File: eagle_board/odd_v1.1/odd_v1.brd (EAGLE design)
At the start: 100 x 40.6 mm, 17 parts

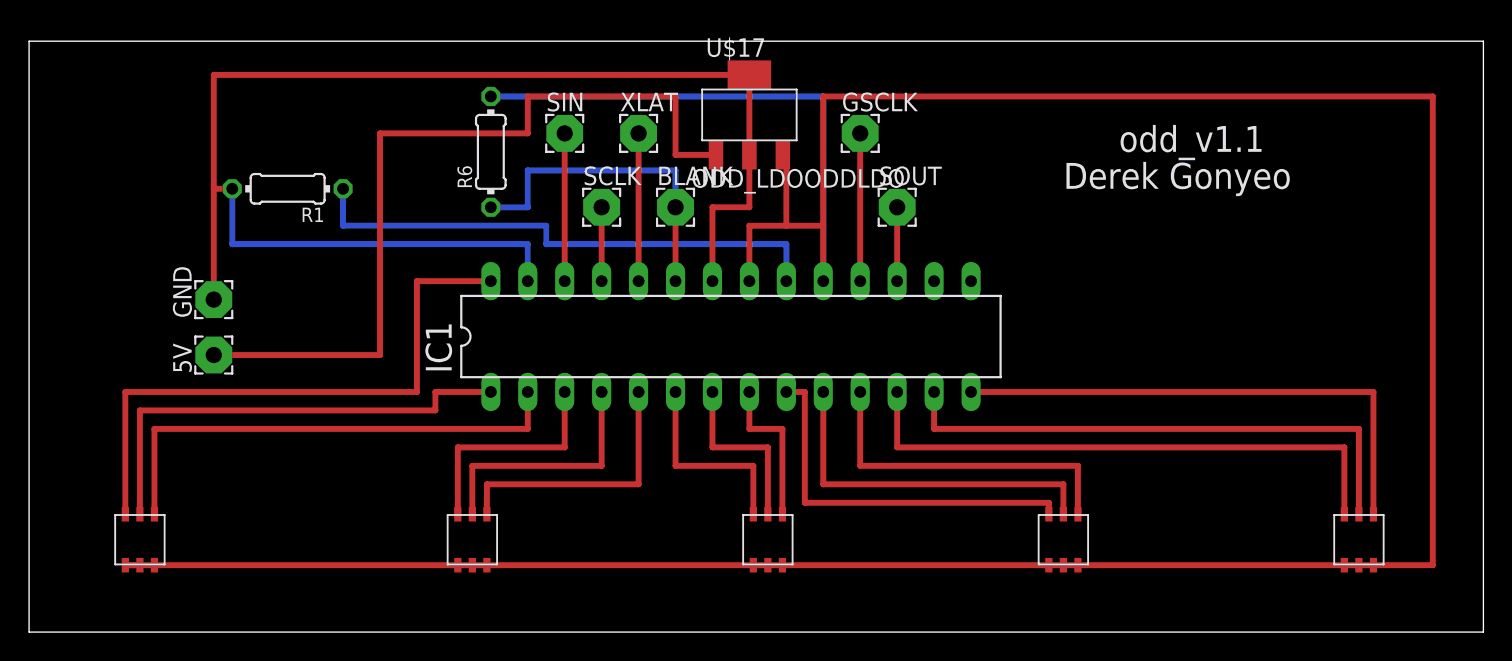
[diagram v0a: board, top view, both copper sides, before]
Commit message: Small changes.
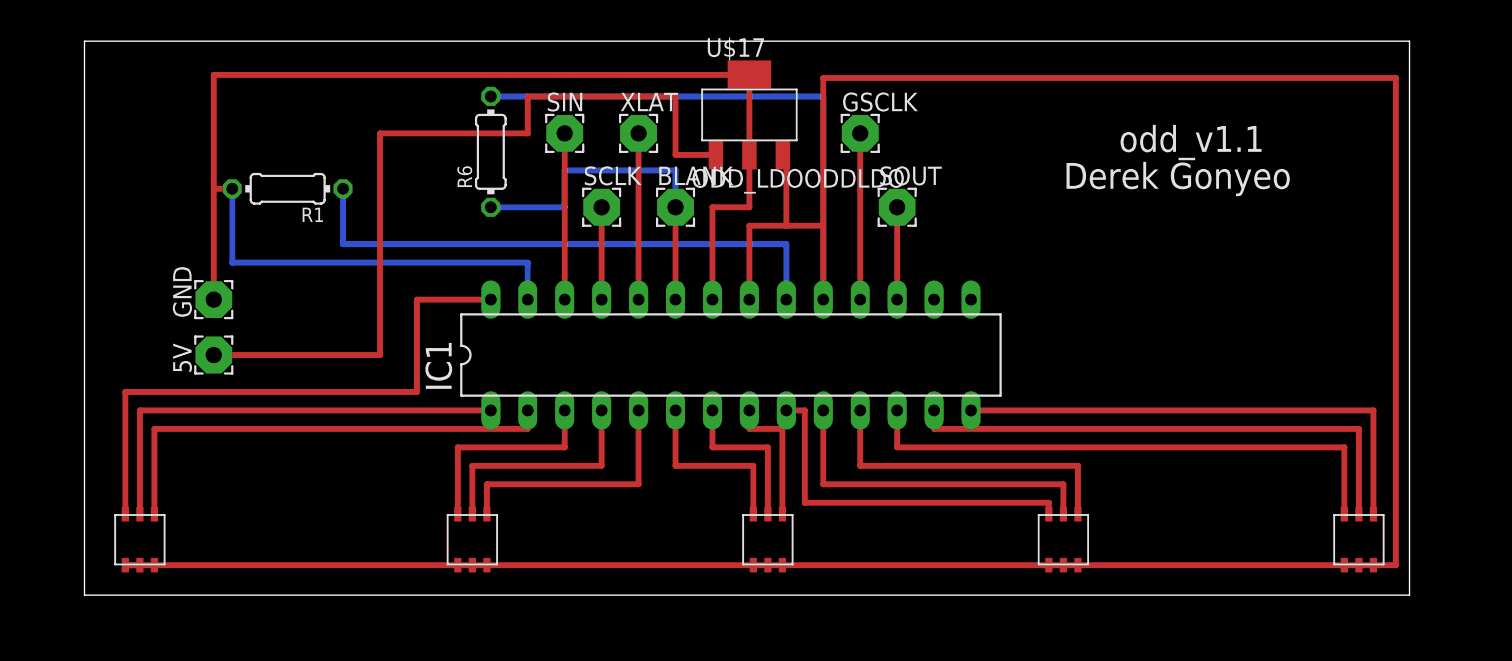
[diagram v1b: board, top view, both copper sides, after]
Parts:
- U$1, U$2, U$3, U$4, U$5: value CREESMDRGBLED6PADSMD -> RGBLED
- moved IC1 1.27 mm to (47.0, 19.1)
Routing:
- net N$19: track 96.9 -> 99.5 mm
- net N$22: track 227.3 -> 228.6 mm
- net N$58: track 36.8 -> 38.1 mm
- net N$16: track 26.5 -> 25.2 mm
- net N$15: track 24.9 -> 23.7 mm
- net N$14: track 23.4 -> 22.1 mm
- net N$13: track 39.2 -> 37.9 mm
- net N$12: track 37.6 -> 36.4 mm
- net N$11: track 36.1 -> 34.8 mm
- net N$1: track 41.2 -> 39.9 mm
- net N$9: track 10.7 -> 9.41 mm
- net N$8: track 12.2 -> 10.9 mm
- net N$7: track 13.8 -> 12.5 mm
- net N$4: track 15.8 -> 14.5 mm
- net N$6: track 18.8 -> 17.6 mm
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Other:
- board size 100 x 40.6 mm -> 91.1 x 38.1 mm
